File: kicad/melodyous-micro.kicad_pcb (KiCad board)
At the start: 2 copper layers, 33.1 x 17.8 mm, 13 parts, among them J1 TRS, U1 ProMicro

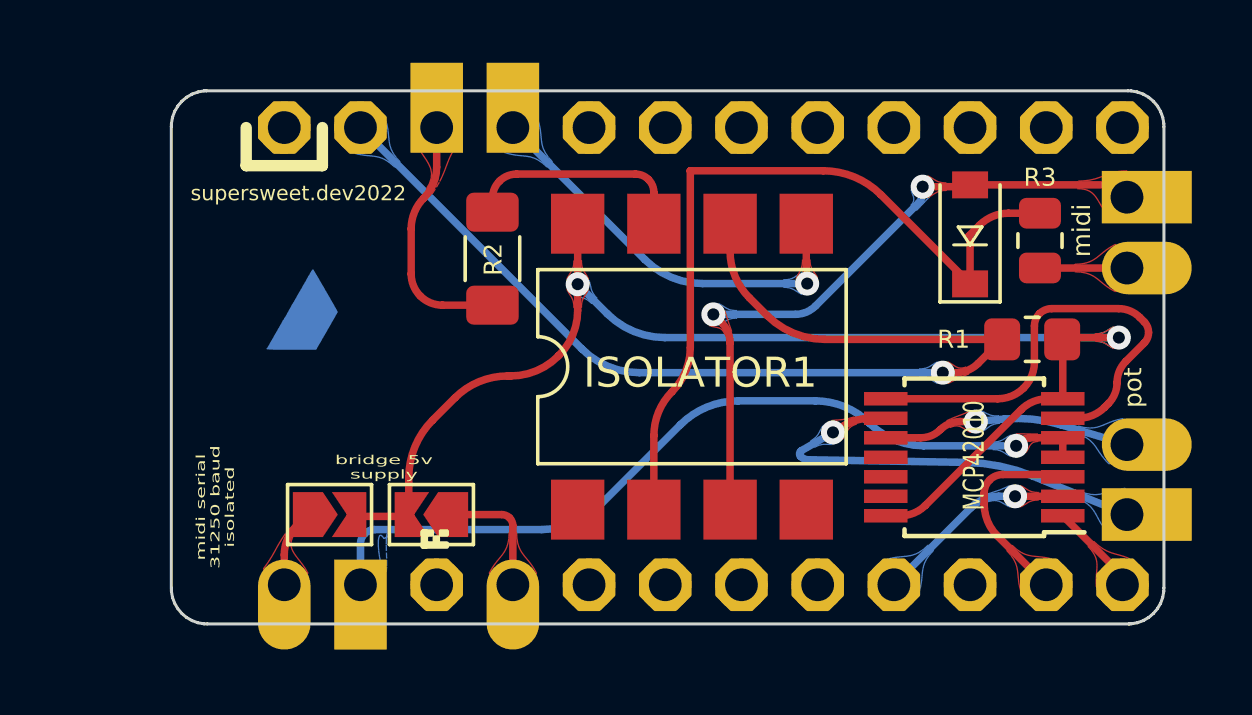
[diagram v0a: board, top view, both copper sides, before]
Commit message: qtpy version
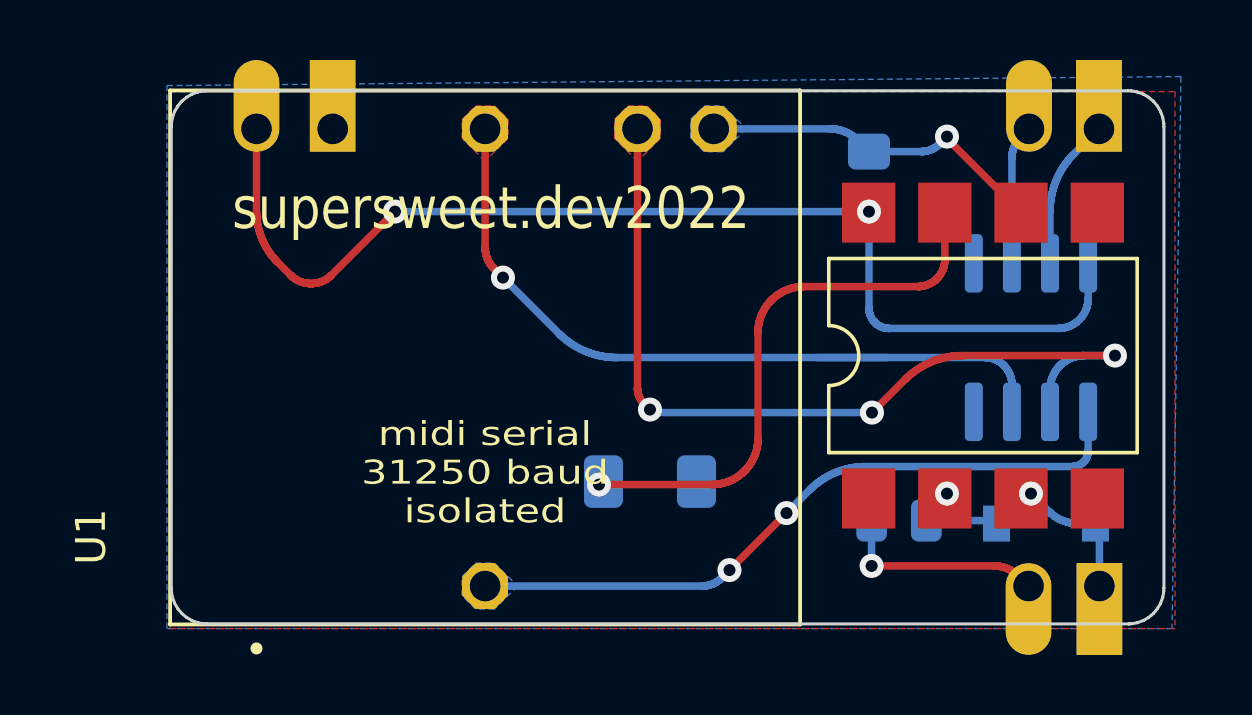
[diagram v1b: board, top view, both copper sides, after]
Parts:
- removed G2***: logo, Keebio-Parts:logo
- removed JP1: RAW5V, Jumper:SolderJumper-2_P1.3mm_Open_TrianglePad1.0x1.5mm
- removed JP2: VCC5V, Jumper:SolderJumper-2_P1.3mm_Open_TrianglePad1.0x1.5mm
- removed MCP42010: MCP42010, Package_SO:TSSOP-14-1EP_4.4x5mm_P0.65mm
- added mcp41010: MCP41010, Package_SO:SOIC-8_3.9x4.9mm_P1.27mm, B.Cu at (132.8, 73.0)
- D1, G***, R1, R2, R3: moved to B.Cu
- POT1: renamed from POTW1; value POT- -> Tape Pot
- U1: value ProMicro -> qtpy; footprint Keebio-Parts:melodyus-controller -> adafruit:qtpy; moved to F.Cu
- moved POT1 12.7 mm to (134.8, 65.9), turned to 90 degrees
- moved J1 12.1 mm to (134.3, 81.2), turned to -90 degrees
- moved R3 10.4 mm to (128.4, 79.1), turned to 0 degrees
- moved D1 9.97 mm to (133.3, 79.2), turned to 0 degrees
- moved ISOLATOR1 9.71 mm to (131.2, 73.6)
- moved R2 9.10 mm to (120.1, 77.8), turned to 0 degrees
- moved R1 7.57 mm to (127.4, 67.8), turned to -90 degrees
- moved U1 7.28 mm to (114.6, 73.7), turned to 90 degrees
- moved G*** 4.97 mm to (114.1, 72.6), turned to 180 degrees
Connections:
- ISOLATOR1 pad 5: Net-(ISOLATOR1-Pad5) -> GND
- ISOLATOR1 pad 8: Net-(ISOLATOR1-Pad8) -> +5V
- R1 pad 2: Net-(ISOLATOR1-Pad8) -> +5V
- R2 pad 2: Net-(ISOLATOR1-Pad5) -> GND
- U1 pad 11: unconnected-(U1-Pad11) -> Net-(U1-Pad11)
- U1 pad 13: Net-(MCP42010-Pad1) -> GND
- U1 pad 14: Net-(MCP42010-Pad3) -> +5V
- U1 pad 4: Net-(ISOLATOR1-Pad5) -> Net-(U1-Pad4)
- U1 pad 8: unconnected-(U1-Pad8) -> Net-(ISOLATOR1-Pad6)
- U1 pad 9: unconnected-(U1-Pad9) -> Net-(U1-Pad9)
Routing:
- net Net-(ISOLATOR1-Pad5): track 49.9 -> 0.00 mm, vias 2 -> 0
- net Net-(ISOLATOR1-Pad8): track 43.1 -> 0.00 mm, vias 2 -> 0
- net +5V: track 0.00 -> 38.2 mm, vias 0 -> 2
- net Net-(U1-Pad9): track 0.00 -> 29.3 mm, vias 0 -> 3
- net Net-(ISOLATOR1-Pad6): track 36.6 -> 11.7 mm
- net Net-(U1-Pad11): track 0.00 -> 24.5 mm, vias 0 -> 1
- net Net-(U1-Pad4): track 0.00 -> 23.2 mm, vias 0 -> 2
- net Net-(D1-Pad1): track 26.6 -> 3.50 mm, vias 0 -> 1
- net Net-(D1-Pad2): track 21.9 -> 4.62 mm, vias 2 -> 1
- net Net-(MCP42010-Pad6): track 15.3 -> 0.00 mm
- net Net-(MCP42010-Pad9): track 14.0 -> 0.00 mm, vias 1 -> 0
- net Net-(ISOLATOR1-Pad7): track 7.21 -> 18.9 mm, vias 0 -> 1
- net Net-(MCP42010-Pad10): track 8.27 -> 0.00 mm, vias 1 -> 0
- net Net-(MCP42010-Pad2): track 6.79 -> 0.00 mm, vias 1 -> 0
- net Net-(MCP42010-Pad3): track 6.73 -> 0.00 mm
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- added copper zone on B.Cu, net GND
- added copper zone on F.Cu, net GND
- added copper zone on B.Cu, net Net-(ISOLATOR1-Pad6)
- added copper zone on F.Cu, net Net-(U1-Pad11)
- added copper zone on B.Cu, net Net-(U1-Pad4)
- added copper zone on F.Cu, net Net-(U1-Pad9)
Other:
- board text added: "QTPY VER."
- board text added: "tape power"
- board text removed: "bridge 5v supply"
